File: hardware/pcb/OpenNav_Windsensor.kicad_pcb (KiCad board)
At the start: 2 copper layers, 5 parts, among them IC1 AS5600-ASOT, U1 XIAO-ESP32-C6, U2 StpDwnE3.3-0.5, U3 SS411P, U4 DS18B20

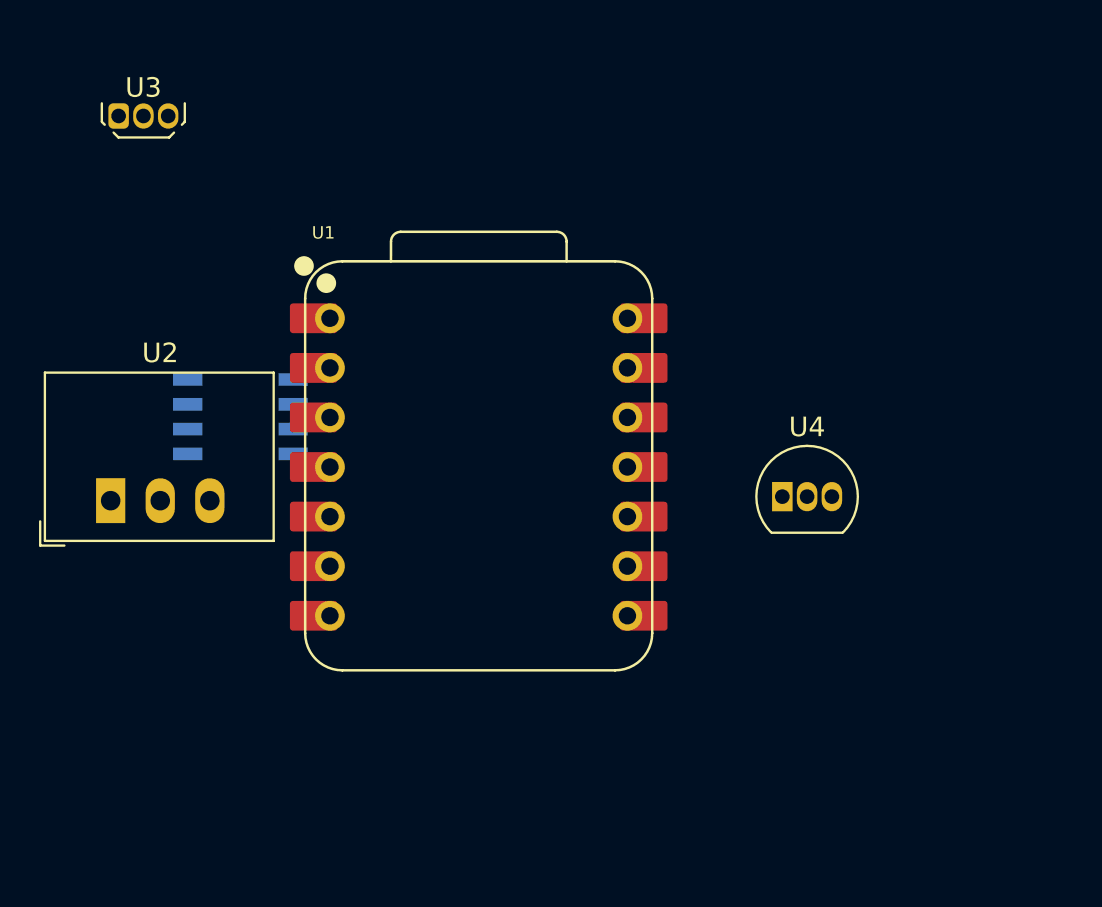
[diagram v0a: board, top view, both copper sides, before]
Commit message: V1
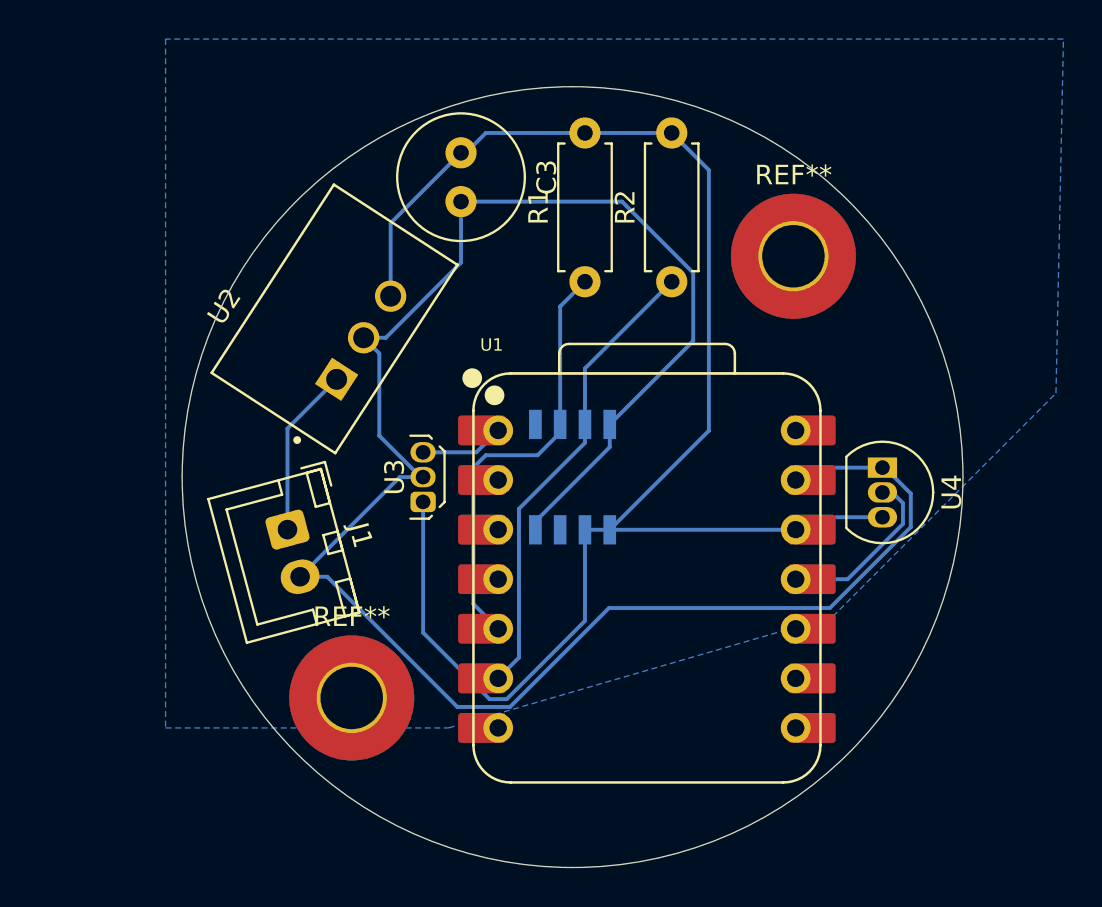
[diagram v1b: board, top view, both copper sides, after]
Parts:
- added C3: 100nF, Capacitor_THT:C_Radial_D6.3mm_H11.0mm_P2.50mm, F.Cu at (127.0, 40.4)
- added J1: Conn_01x02_Pin, Connector_JST:JST_XH_B2B-XH-A_1x02_P2.50mm_Vertical, F.Cu at (118.1, 59.7)
- added R1: 5k, Resistor_THT:R_Axial_DIN0207_L6.3mm_D2.5mm_P7.62mm_Horizontal, F.Cu at (133.3, 47.0)
- added R2: 5k, Resistor_THT:R_Axial_DIN0207_L6.3mm_D2.5mm_P7.62mm_Horizontal, F.Cu at (137.8, 47.0)
- added REF**: MountingHole_3.2mm_M3_Pad_TopBottom, MountingHole:MountingHole_3.2mm_M3_Pad_TopBottom, F.Cu at (121.4, 68.3)
- added REF**: MountingHole_3.2mm_M3_Pad_TopBottom, MountingHole:MountingHole_3.2mm_M3_Pad_TopBottom, F.Cu at (144.0, 45.7)
- U2: footprint Converter_DCDC:Converter_DCDC_RECOM_R-78E-0.5_THT -> Custom:CONV_R-78K3.3-0.5
- U3: footprint Package_TO_SOT_THT:TO-92Flat -> Custom:SS411P
- moved U3 25.2 mm to (125.1, 58.3), turned to 90 degrees
- moved IC1 17.3 mm to (132.7, 57.0), turned to 90 degrees
- moved U2 14.8 mm to (120.5, 48.9), turned to 57 degrees
- moved U1 10.4 mm to (136.6, 62.2)
- moved U4 5.34 mm to (148.6, 56.5), turned to -90 degrees
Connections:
- U1 pad 1: unconnected-(U1-GPIO0/A0/D0-Pad1) -> Net-(U1-GPIO0/A0/D0)
- U1 pad 10: Net-(U1-GPIO20/D9/MISO) -> unconnected-(U1-GPIO20/D9/MISO-Pad10)
- U1 pad 11: unconnected-(U1-GPIO18/D10/MOSI-Pad11)_1 -> Net-(U1-GPIO18/D10/MOSI)
- U1 pad 8: Net-(U1-GPIO17/D7/RX) -> unconnected-(U1-GPIO17/D7/RX-Pad8)
- U3 pad 3: Net-(U1-GPIO20/D9/MISO) -> Net-(U1-GPIO0/A0/D0)
- U4 pad 2: Net-(U1-GPIO17/D7/RX) -> Net-(U1-GPIO18/D10/MOSI)
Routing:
- net GND: track 0.00 -> 102.8 mm
- net +3.3V: track 0.00 -> 81.5 mm
- net Net-(IC1-SCL): track 0.00 -> 24.0 mm
- net Net-(IC1-SDA): track 0.00 -> 22.2 mm
- net Net-(U1-GPIO18/D10/MOSI): track 0.00 -> 9.01 mm
- net VCC: track 0.00 -> 8.74 mm
- net Net-(U1-GPIO0/A0/D0): track 0.00 -> 4.31 mm
- added copper zone on B.Cu, net GND
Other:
- board outline added: 40 x 40 mm
